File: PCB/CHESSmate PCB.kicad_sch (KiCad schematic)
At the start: 52 parts, among them J1 Conn_01x20_Pin, J2 Piezo Speaker, Q1 2N2222, Q2 2N2222, Q3 2N2222, Q4 2N2222, SW1 A, SW10 2, SW11 3, SW12 4, SW13 5, SW14 6, SW15 7, SW16 8, SW17 NEW GAME, SW18 CLEAR, SW19 ENTER, SW2 B, SW3 C, SW4 D, SW5 E, SW6 F, SW7 G, SW8 H, SW9 1, U1 SEG 1, U2 SEG 2, U3 SEG 3, U4 SEG 4

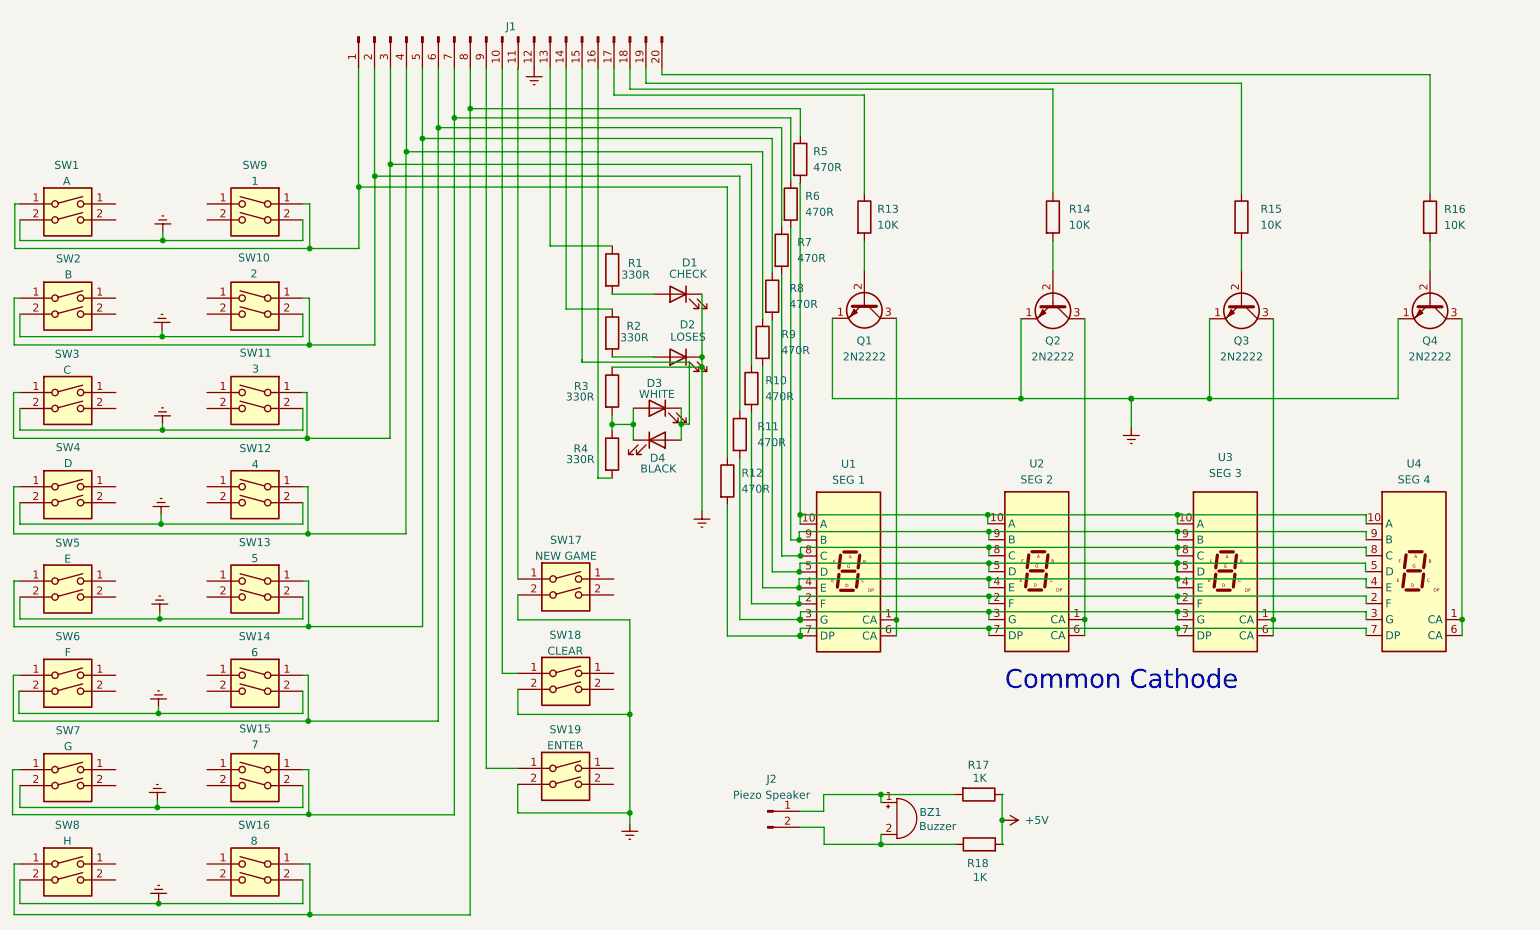
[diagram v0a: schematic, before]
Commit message: Add files via upload
Updated to latest version of schematic.
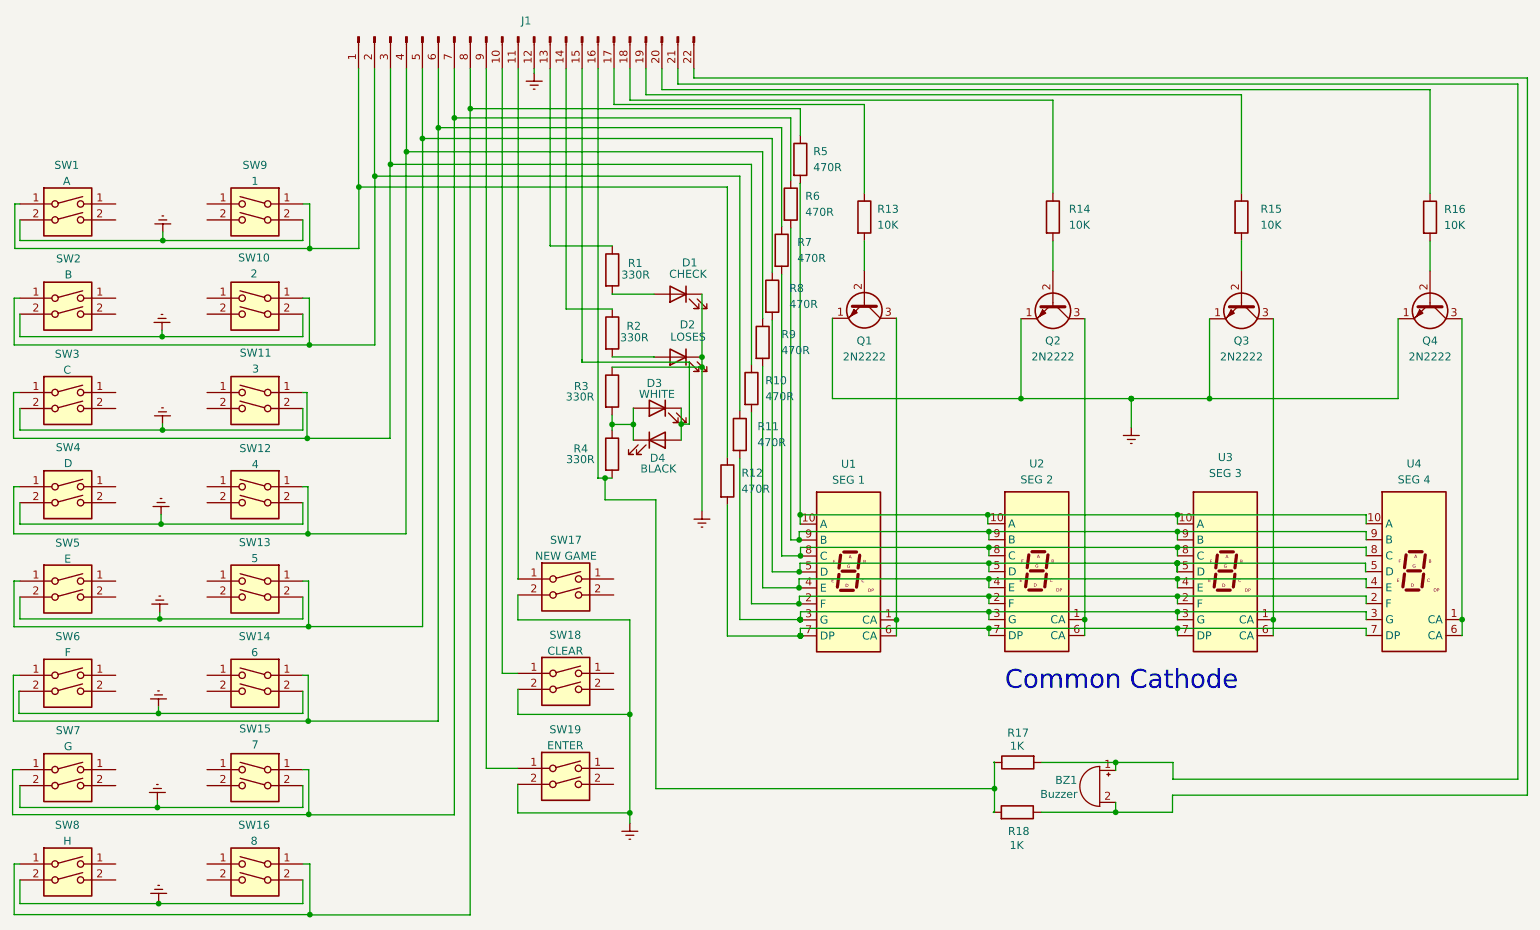
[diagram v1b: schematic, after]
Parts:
- removed J1: Conn_01x20_Pin, Connector_PinHeader_2.54mm:PinHeader_1x20_P2.54mm_Vertical, symbol Connector:Conn_01x20_Pin
- removed J2: Piezo Speaker, symbol Connector:Conn_01x02_Pin
- added J1: Conn_01x22_Pin, symbol Connector:Conn_01x22_Pin
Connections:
- net +5V is gone; now on an unnamed net: R17.1, R18.2
- net GNDREF: now also J1.12 (Pin_12)
- net at D3.1 (K), D4.2 (A): now also J1.15 (Pin_15)
- net at SW11.1: now also R10.1, SW3.1, J1.3 (Pin_3)
- net at R1.1: now also J1.13 (Pin_13)
- net at SW17.1: now also J1.11 (Pin_11)
- net at R2.1: now also J1.14 (Pin_14)
- net at SW9.1: now also R12.1, SW1.1, J1.1 (Pin_1)
- net at BZ1.2 (+), R18.1: now also J1.22 (Pin_22)
- net at SW18.1: now also J1.10 (Pin_10)
- net at R16.1: now also J1.20 (Pin_20)
- net at SW14.1: now also R7.1, SW6.1, J1.6 (Pin_6)
- net at R14.1: now also J1.18 (Pin_18)
- net at BZ1.1 (-), R17.2: now also J1.21 (Pin_21)
- net at R15.1: now also J1.19 (Pin_19)
- net at SW19.1: now also J1.9 (Pin_9)
- net at R4.2: now also J1.16 (Pin_16)
- net at R13.1: now also J1.17 (Pin_17)
- net at R6.1, SW15.1, SW7.1: now also J1.7 (Pin_7)
- net at R5.1, SW16.1, SW8.1: now also J1.8 (Pin_8)
- new net: J1.2 (Pin_2), R11.1, SW10.1, SW2.1
- new net: J1.5 (Pin_5), R8.1, SW13.1, SW5.1
- new net: J1.4 (Pin_4), R9.1, SW12.1, SW4.1
- now unconnected: SW1.1, SW10.1, SW12.1, SW13.1, SW2.1, SW3.1, SW4.1, SW5.1, SW6.1
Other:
- moved on the sheet: BZ1, R17, R18
